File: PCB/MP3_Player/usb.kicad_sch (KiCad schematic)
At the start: 13 parts, among them J2 USB_C_Receptacle, J3 USB_A, U4 TS3USB30ERSWR

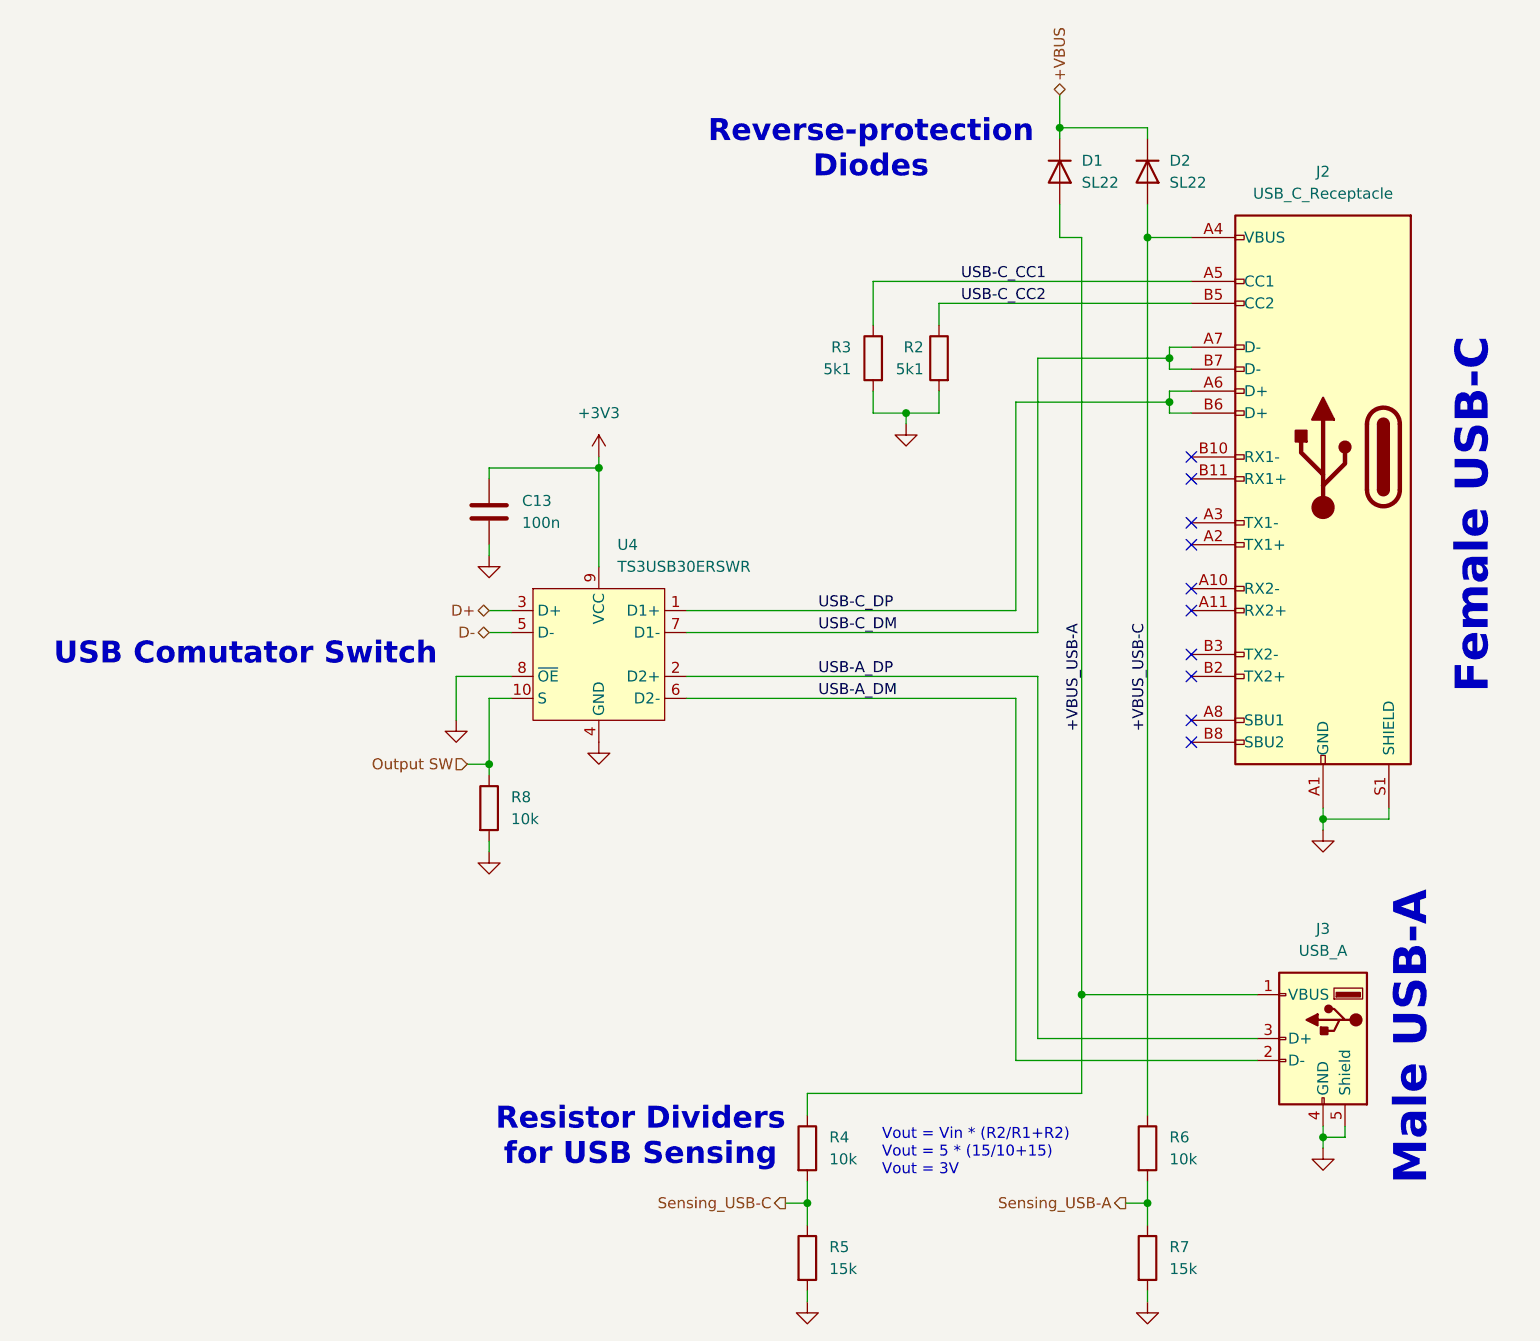
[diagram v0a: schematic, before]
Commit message: Continue Making BOM
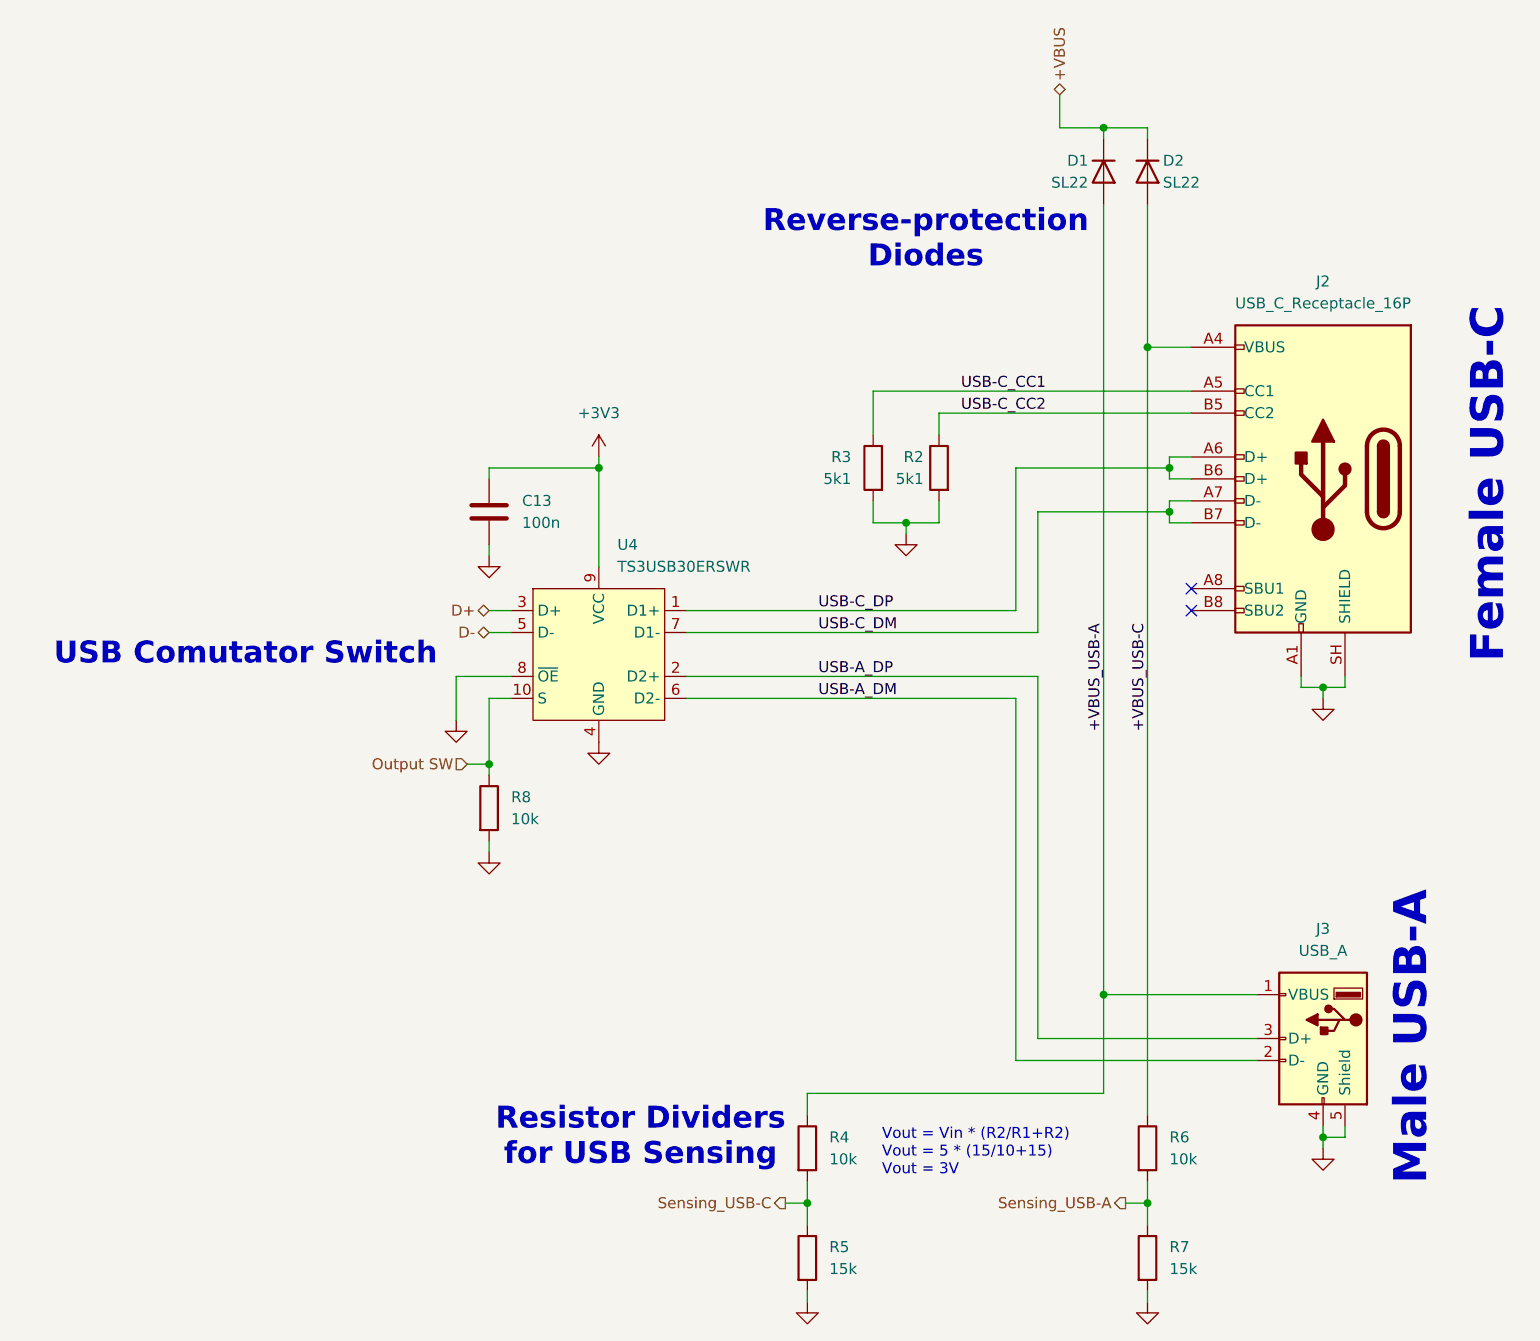
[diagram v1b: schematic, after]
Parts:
- removed J2: USB_C_Receptacle, symbol Connector:USB_C_Receptacle
- added J2: USB_C_Receptacle_16P, symbol Connector:USB_C_Receptacle_USB2.0_16P
- R2, R3: Mfr. Part # (none) -> CRCW04025K10FKED; Store URL - Digikey (none) -> https://www.digikey.pt/pt/products/detail/vishay-dale/CRCW0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; Store URL - Mouser (none) -> https://pt.mouser.com/en/ProductDetail/Vishay/CRCW04025K10F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
- R4, R6, R8: Mfr. Part # (none) -> CRCW040210K0FKED; Store URL - Digikey (none) -> https://www.digikey.pt/pt/products/detail/vishay-dale/CRCW0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; Store URL - Mouser (none) -> https://pt.mouser.com/en/ProductDetail/Vishay/CRCW040210K0F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
- R5, R7: Mfr. Part # (none) -> CRCW040215K0FKED; Store URL - Digikey (none) -> https://www.digikey.pt/pt/products/detail/vishay-dale/CRCW0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; Store URL - Mouser (none) -> https://pt.mouser.com/en/ProductDetail/Vishay/CRCW040215K0F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
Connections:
- net +VBUS_USB-C: now also J2.A4 (VBUS), J2.A9 (VBUS), J2.B4 (VBUS), J2.B9 (VBUS)
- net GND: now also J2.A1 (GND), J2.A12 (GND), J2.B1 (GND), J2.B12 (GND), J2.SH (SHIELD)
- net USB-C_CC1: now also J2.A5 (CC1)
- net USB-C_CC2: now also J2.B5 (CC2)
- net USB-C_DM: now also J2.A7 (D-), J2.B7 (D-)
- net USB-C_DP: now also J2.A6 (D+), J2.B6 (D+)
- no-connect marks 10 -> 2
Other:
- moved on the sheet: D1, R2, R3
